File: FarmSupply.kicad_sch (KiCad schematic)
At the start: 12 parts, among them P1 USB_C_Plug, P2 USB_C_Plug, P3 USB_C_Plug, P4 USB_C_Plug, P5 USB_C_Plug, P6 USB_C_Plug

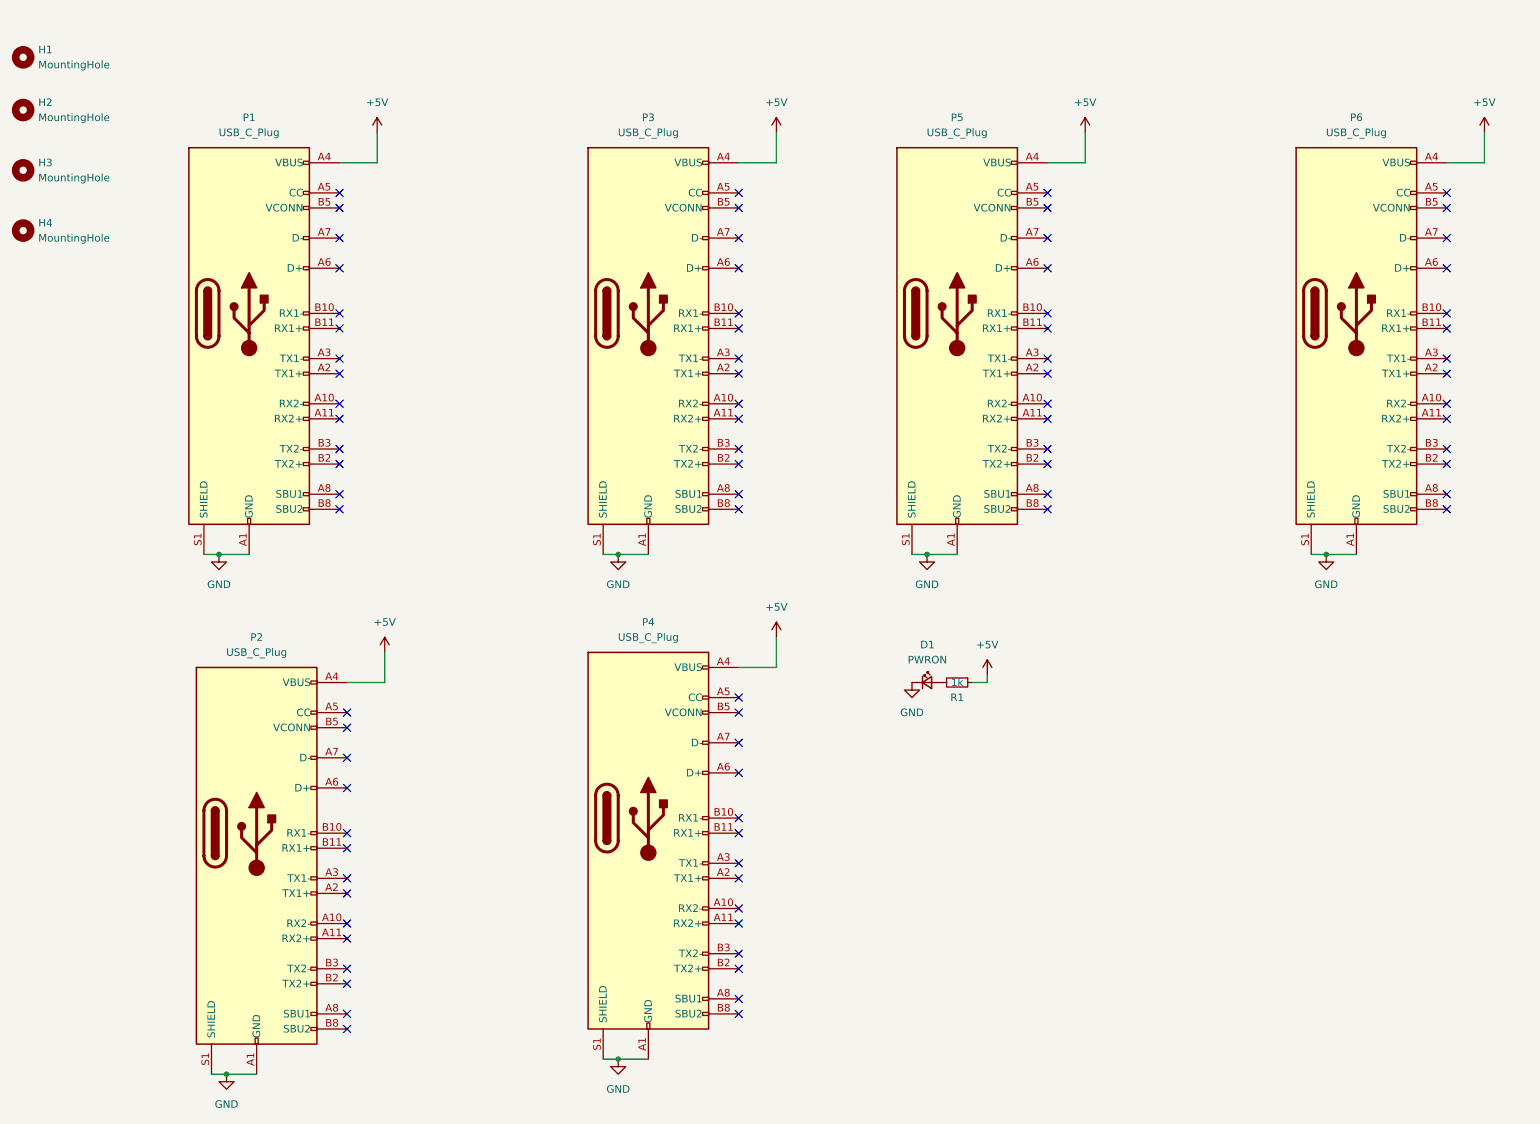
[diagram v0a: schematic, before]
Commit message: Add files via upload
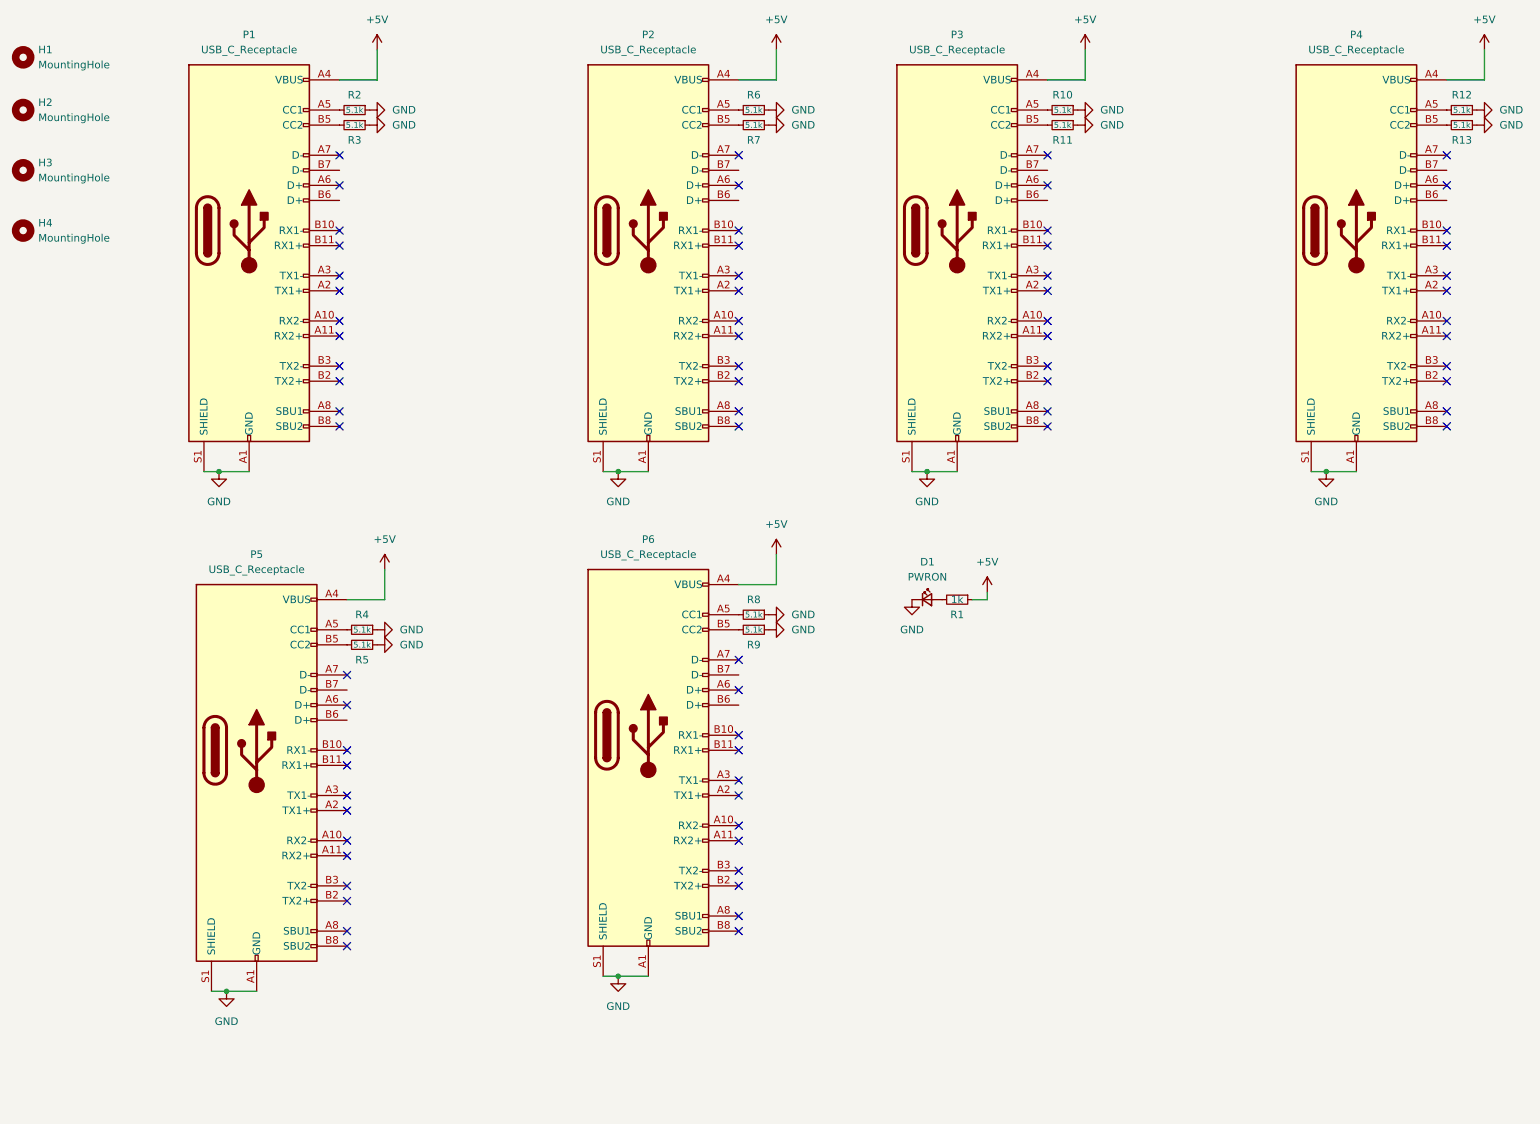
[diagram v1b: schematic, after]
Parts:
- removed P1, P2, P3, P4, P5, P6: USB_C_Plug, 18650:GT-USB-7010, symbol Connector:USB_C_Plug
- added P1, P2, P3, P4, P5, P6: USB_C_Receptacle, 18650:GT-USB-7010, symbol Connector:USB_C_Receptacle
- added R10, R11, R12, R13, R2, R3, R4, R5, R6, R7, R8, R9: 5.1k, Resistor_SMD:R_0805_2012Metric, symbol Device:R_Small
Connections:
- net +5V: now also P1.A4 (VBUS), P1.A9 (VBUS), P1.B4 (VBUS), P1.B9 (VBUS), P2.A4 (VBUS), P2.A9 (VBUS), P2.B4 (VBUS), P2.B9 (VBUS), P3.A4 (VBUS), P3.A9 (VBUS), P3.B4 (VBUS), P3.B9 (VBUS), P4.A4 (VBUS), P4.A9 (VBUS), P4.B4 (VBUS), P4.B9 (VBUS), P5.A4 (VBUS), P5.A9 (VBUS), P5.B4 (VBUS), P5.B9 (VBUS), P6.A4 (VBUS), P6.A9 (VBUS), P6.B4 (VBUS), P6.B9 (VBUS)
- net GND: now also P1.A1 (GND), P1.A12 (GND), P1.B1 (GND), P1.B12 (GND), P1.S1 (SHIELD), P2.A1 (GND), P2.A12 (GND), P2.B1 (GND), P2.B12 (GND), P2.S1 (SHIELD), P3.A1 (GND), P3.A12 (GND), P3.B1 (GND), P3.B12 (GND), P3.S1 (SHIELD), P4.A1 (GND), P4.A12 (GND), P4.B1 (GND), P4.B12 (GND), P4.S1 (SHIELD), P5.A1 (GND), P5.A12 (GND), P5.B1 (GND), P5.B12 (GND), P5.S1 (SHIELD), P6.A1 (GND), P6.A12 (GND), P6.B1 (GND), P6.B12 (GND), P6.S1 (SHIELD), R10.1, R11.1, R12.1, R13.1, R2.1, R3.1, R4.1, R5.1, R6.1, R7.1, R8.1, R9.1
- new net: P2.A5 (CC1), R6.2
- new net: P6.A5 (CC1), R8.2
- new net: P6.B5 (CC2), R9.2
- new net: P3.B5 (CC2), R11.2
- new net: P4.A5 (CC1), R12.2
- new net: P4.B5 (CC2), R13.2
- new net: P1.A5 (CC1), R2.2
- new net: P1.B5 (CC2), R3.2
- new net: P3.A5 (CC1), R10.2
- new net: P2.B5 (CC2), R7.2
- new net: P5.A5 (CC1), R4.2
- new net: P5.B5 (CC2), R5.2
- no-connect marks 84 -> 72
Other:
- moved on the sheet: D1, R1
